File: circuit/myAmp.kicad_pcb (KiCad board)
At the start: 2 copper layers, 66 x 72 mm, 49 parts, among them J1 JACK_MONO, J2 HOLE, J3 HOLE, J4 HOLE, J5 HOLE, Q1 J201, Q2 J201, U1 TPA3136D2

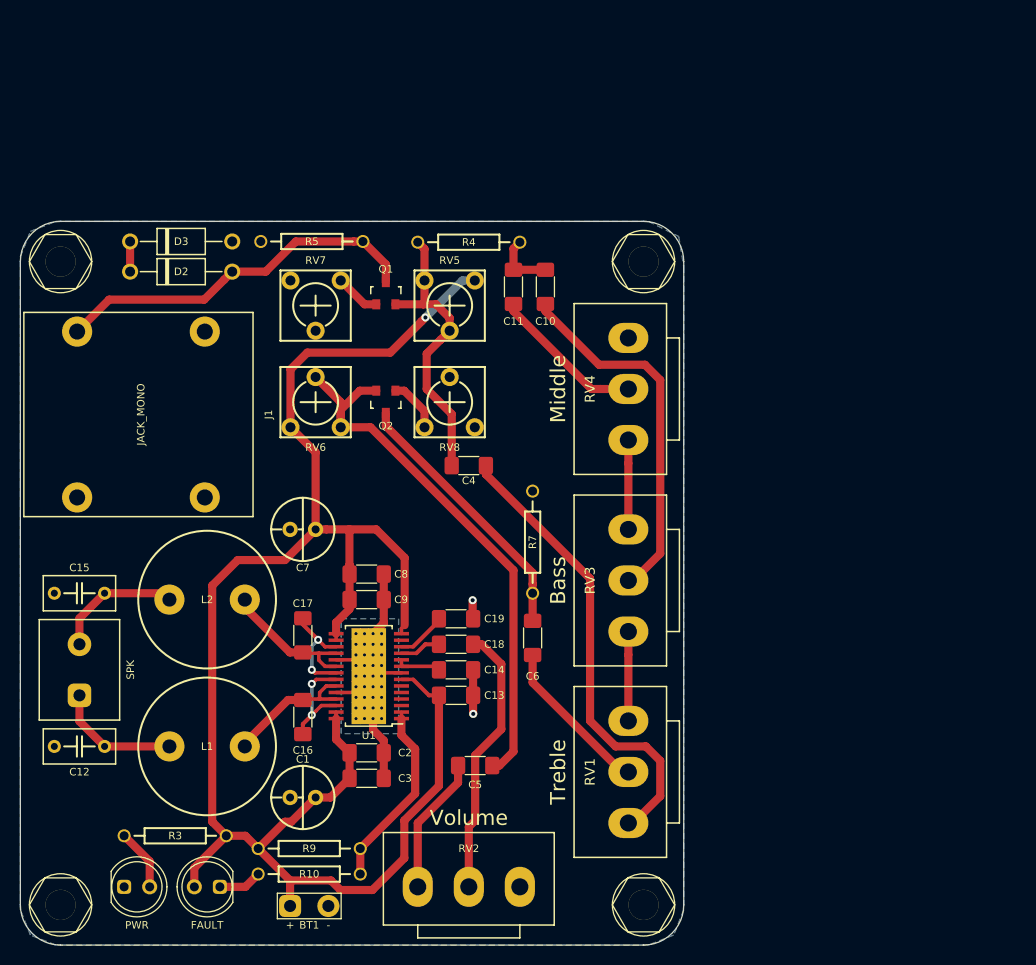
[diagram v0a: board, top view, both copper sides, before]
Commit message: modular version in beta
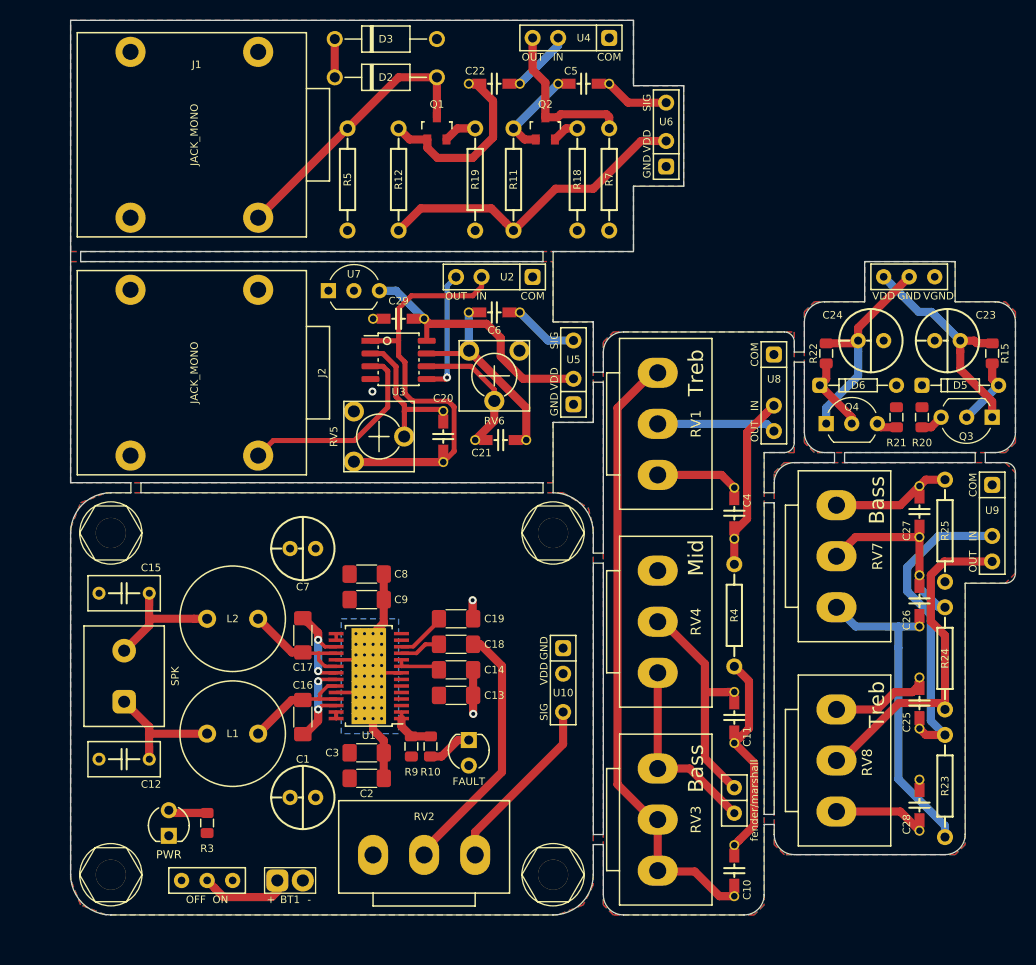
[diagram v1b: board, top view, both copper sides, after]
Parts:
- added C20: 1nF, myAmp:C_5MM, F.Cu at (92.1, 71.4)
- added C21: 1nF, myAmp:C_5MM, F.Cu at (97.8, 71.8)
- added C22: 100nF, myAmp:C_5MM, F.Cu at (97.2, 36.3)
- added C23: 220μF, myAmp:CPOL_D6.3_P2.5, F.Cu at (142.2, 61.9)
- added C24: 220μF, myAmp:CPOL_D6.3_P2.5, F.Cu at (134.6, 61.9)
- added C25: 330pF, myAmp:C_5MM, F.Cu at (139.4, 97.9)
- added C26: 470pF, myAmp:C_5MM, F.Cu at (139.4, 87.8)
- added C27: 4.7nF, myAmp:C_5MM, F.Cu at (139.4, 78.9)
- added C28: 2.2nF, myAmp:C_5MM, F.Cu at (139.4, 108.1)
- added C29: 100nF, myAmp:C_5MM, F.Cu at (87.6, 59.7)
- added D5: 1N4148, myAmp:DO35, F.Cu at (143.5, 66.3)
- added D6: 1N4148, myAmp:DO35, F.Cu at (133.3, 66.3)
- added J6: HOLE, myAmp:MountingHole, F.Cu at (103.0, 81.0)
- added J7: CONN_01X03, myAmp:SPLITTER, F.Cu at (138.4, 55.5)
- added Q3: BC547, myAmp:TO-92_Inline_Wide, F.Cu at (144.1, 69.5)
- added Q4: BC557, myAmp:TO-92_Inline_Wide, F.Cu at (132.7, 70.1)
- added R11: 1, myAmp:R_10MM, F.Cu at (99.1, 45.8)
- added R12: 1, myAmp:R_10MM, F.Cu at (87.6, 45.8)
- added R15: 4K7, myAmp:R_0805, F.Cu at (146.7, 63.1)
- added R18: 1, myAmp:R_10MM, F.Cu at (105.4, 45.8)
- added R19: 1, myAmp:R_10MM, F.Cu at (95.2, 45.8)
- added R20: 10, myAmp:R_0805, F.Cu at (139.7, 69.5)
- added R21: 10, myAmp:R_0805, F.Cu at (137.2, 69.5)
- added R22: 4K7, myAmp:R_0805, F.Cu at (130.2, 63.1)
- added R23: 100K, myAmp:R_10MM, F.Cu at (142.0, 106.2)
- added R24: 180K, myAmp:R_10MM, F.Cu at (142.0, 93.5)
- added R25: 10K, myAmp:R_10MM, F.Cu at (142.0, 80.8)
- added SW1: OFF ON, myAmp:SW_TINY, F.Cu at (68.6, 115.6)
- added SW2: fender/marshall, myAmp:JUMPER, F.Cu at (121.0, 107.6)
- added U10: PREAMP_CON, myAmp:PREAMP_CON, F.Cu at (104.0, 95.0)
- added U2: TONE_CON, myAmp:TONE_CON, F.Cu at (97.2, 55.5)
- added U3: TL072, myAmp:SOIC-8_3.9x4.9mm_P1.27mm, F.Cu at (87.6, 63.8)
- added U4: TONE_CON, myAmp:TONE_CON, F.Cu at (104.8, 31.8)
- added U5: PREAMP_CON, myAmp:PREAMP_CON, F.Cu at (105.0, 65.7)
- added U6: PREAMP_CON, myAmp:PREAMP_CON, F.Cu at (114.2, 42.0)
- added U7: TLE2426, myAmp:TO-92_Inline_Wide, F.Cu at (83.2, 56.9)
- added U8: TONE_CON, myAmp:TONE_CON, F.Cu at (125.0, 67.1)
- added U9: TONE_CON, myAmp:TONE_CON, F.Cu at (146.7, 80.0)
- C10, C11, C4: footprint myAmp:C_1206 -> myAmp:C_5MM
- C13, C14, C18, C19: value 1uF -> 1μF
- C5, C6: value 47nF -> 100nF; footprint myAmp:C_1206 -> myAmp:C_5MM
- D1, D4: footprint myAmp:LED_D5.0mm -> myAmp:LED_D3.0mm
- J2: value HOLE -> JACK_MONO; footprint myAmp:MountingHole -> myAmp:JACK_CL13106
- L1, L2: footprint myAmp:COILCRAFT_RFS1412 -> myAmp:COILCRAFT_DR0810
- Q1, Q2: value J201 -> MMBFJ201
- R10, R3, R9: footprint myAmp:R_10MM -> myAmp:R_0805
- RV7: value 2K -> 500K; footprint myAmp:RPOT_RKT6V -> myAmp:POT_VULGARIS
- RV8: value 50K -> 250K; footprint myAmp:RPOT_RKT6V -> myAmp:POT_VULGARIS
- moved J2 69.3 mm to (67.3, 65.1), turned to 90 degrees
- moved C5 68.7 mm to (106.0, 36.3), turned to 180 degrees
- moved J5 61.7 mm to (103.0, 115.0)
- moved C10 61.0 mm to (121.0, 114.6)
- moved RV7 58.6 mm to (131.2, 83.3), turned to 270 degrees
- moved RV8 50.8 mm to (131.2, 103.6), turned to 270 degrees
- moved C11 48.1 mm to (121.0, 99.4), turned to 270 degrees
- moved R4 45.6 mm to (121.0, 89.2), turned to 90 degrees
- moved R7 36.9 mm to (108.6, 45.8), turned to 270 degrees
- moved RV1 34.8 mm to (113.4, 70.1), turned to 270 degrees
- moved C6 32.6 mm to (97.2, 59.1), turned to 180 degrees
- moved Q2 31.5 mm to (102.2, 40.8), turned to 0 degrees
- moved D4 29.3 mm to (94.6, 102.9), turned to 90 degrees
- moved D3 28.6 mm to (86.4, 31.9)
- moved J1 28.3 mm to (67.3, 41.4)
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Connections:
- net Net-(D2-Pad2) renamed /guit1
- net PREAMP_OUT renamed Net-(C18-Pad2)
- BT1 pad 1: VDD -> Net-(BT1-Pad1)
- C4 pad 2: /TONE_IN -> Net-(C4-Pad2)
- C6 pad 1: /TONE_OUT -> Net-(C6-Pad1)
- C6 pad 2: Net-(C6-Pad2) -> Net-(C21-Pad1)
- J2 pad 1: Net-(J2-Pad1) -> VGND
- J3 pad 1: Net-(J3-Pad1) -> (no net)
- J4 pad 1: Net-(J4-Pad1) -> (no net)
- J5 pad 1: Net-(J5-Pad1) -> (no net)
- Q1 pad 1: Net-(Q1-Pad1) -> Net-(C22-Pad2)
- Q1 pad 2: /TONE_IN -> Net-(Q1-Pad2)
- Q2 pad 1: Net-(Q2-Pad1) -> Net-(C5-Pad2)
- Q2 pad 2: Net-(C5-Pad2) -> Net-(Q2-Pad2)
- Q2 pad 3: /TONE_OUT -> Net-(Q2-Pad3)
- R4 pad 2: /TONE_IN -> Net-(C4-Pad2)
- R7 pad 1: /TONE_OUT -> Net-(Q2-Pad3)
- RV1 pad 1: Net-(C4-Pad1) -> Net-(C10-Pad1)
- RV1 pad 2: Net-(C6-Pad2) -> Net-(RV1-Pad2)
- RV1 pad 3: Net-(RV1-Pad3) -> Net-(C4-Pad1)
- RV2 pad 1: Net-(C5-Pad1) -> GND
- RV2 pad 3: GND -> Net-(RV2-Pad3)
- RV3 pad 1: Net-(RV1-Pad3) -> Net-(RV3-Pad1)
- RV3 pad 3: Net-(RV3-Pad3) -> Net-(C10-Pad1)
- RV4 pad 1: Net-(RV3-Pad3) -> GND
- RV4 pad 3: GND -> Net-(RV3-Pad1)
- RV5 pad 1: VDD -> VGND
- RV5 pad 2: /TONE_IN -> Net-(C20-Pad2)
- RV5 pad 3: /TONE_IN -> Net-(C20-Pad1)
- RV6 pad 1: VDD -> VGND
- RV6 pad 2: Net-(C5-Pad2) -> Net-(C21-Pad2)
- RV6 pad 3: Net-(C5-Pad2) -> Net-(C21-Pad1)
- RV7 pad 1: Net-(Q1-Pad1) -> Net-(C27-Pad1)
- RV7 pad 2: GND -> Net-(C26-Pad1)
- RV7 pad 3: GND -> Net-(C26-Pad2)
- RV8 pad 1: Net-(Q2-Pad1) -> Net-(C25-Pad2)
- RV8 pad 2: GND -> Net-(R24-Pad2)
- RV8 pad 3: GND -> Net-(C28-Pad1)
- U1 pad 13: Net-(U1-Pad13) -> (no net)
- U1 pad 3: Net-(U1-Pad3) -> (no net)
- U1 pad 4: Net-(U1-Pad4) -> (no net)
- U1 pad 5: Net-(U1-Pad5) -> (no net)
- U1 pad 6: Net-(U1-Pad6) -> (no net)
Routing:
- net VDD: track 177.7 -> 83.3 mm, vias 1 -> 0
- net Net-(C5-Pad2): track 55.9 -> 9.91 mm
- net Net-(C20-Pad1): track 0.00 -> 42.9 mm
- net Net-(C4-Pad1): track 46.1 -> 9.09 mm
- net Net-(R24-Pad2): track 0.00 -> 34.0 mm
- net Net-(C26-Pad2): track 0.00 -> 32.8 mm
- net Net-(C25-Pad1): track 0.00 -> 31.7 mm
- net /TONE_IN: track 29.1 -> 0.00 mm
- net /TONE_OUT: track 26.7 -> 0.00 mm
- net Net-(C10-Pad1): track 36.5 -> 63.0 mm
- net GND: track 28.8 -> 51.0 mm, vias 2 -> 3
- net Net-(C21-Pad1): track 0.00 -> 21.3 mm
- net /guit2: track 0.00 -> 20.4 mm
- net Net-(C26-Pad1): track 0.00 -> 19.3 mm
- net Net-(RV3-Pad1): track 0.00 -> 19.0 mm
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- added copper zone on F.Cu, net GND
- added copper zone on F.Cu, net VDD
- added copper zone on B.Cu, net VGND
- added copper zone on F.Cu, net VGND
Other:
- board size 66 x 72 mm -> 94 x 89 mm
- board text added: "2020 apr 29"
- board text added: "GND"
- board text added: "Mid"
- board text added: "Treb"
- board text added: "VDD"
- board text added: "VGND"
- board text removed: "Middle"
- board text removed: "Treble"
- board text removed: "Volume"
